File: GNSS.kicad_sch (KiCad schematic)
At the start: 0 parts

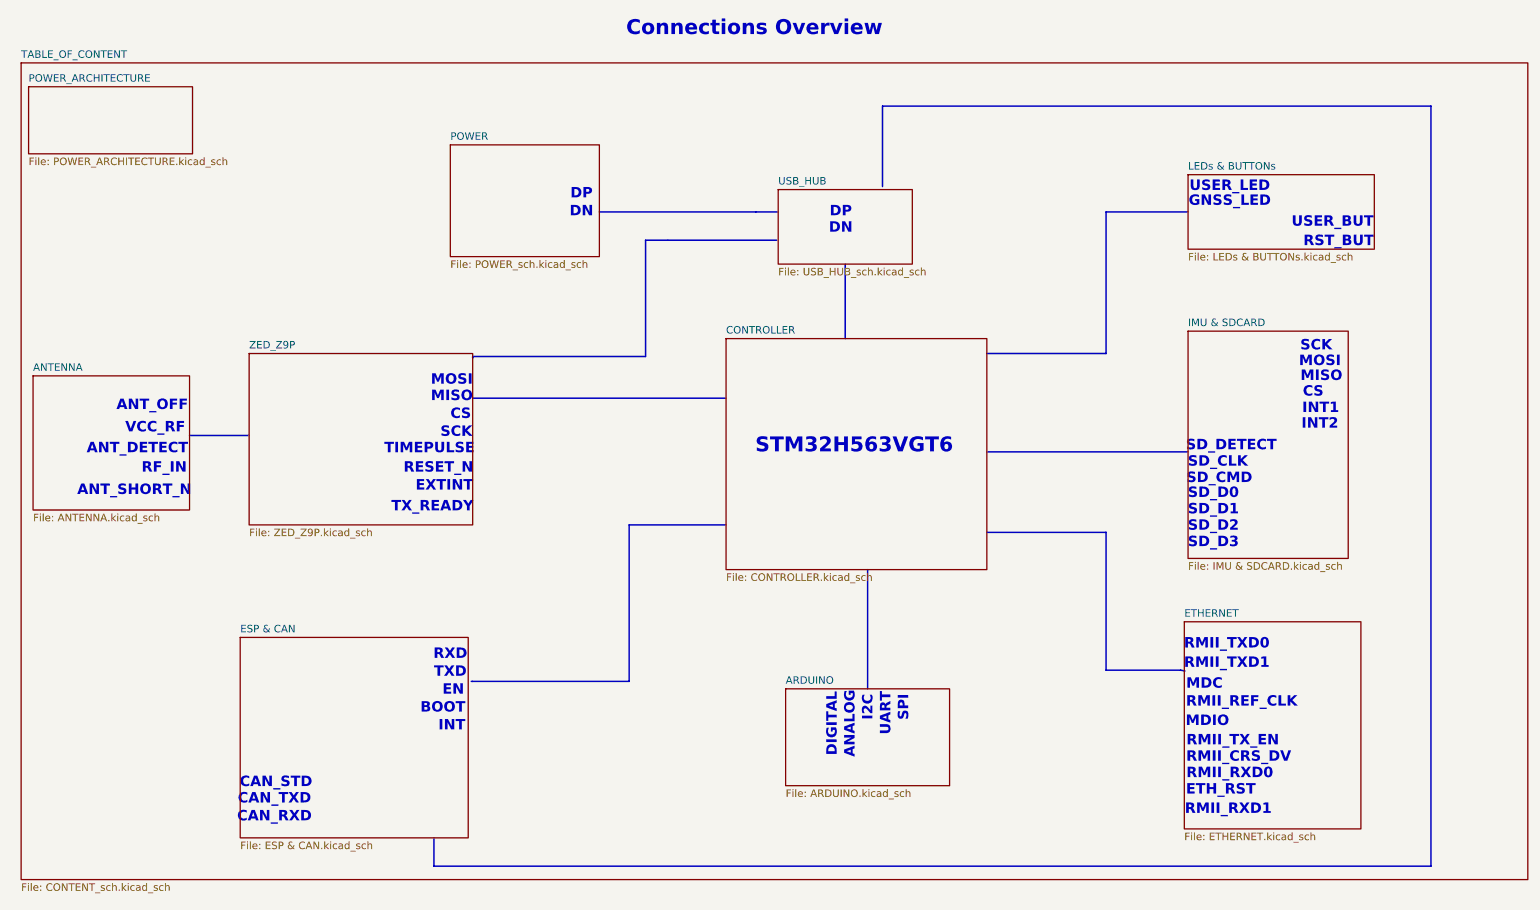
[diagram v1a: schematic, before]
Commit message: 18.09.2026
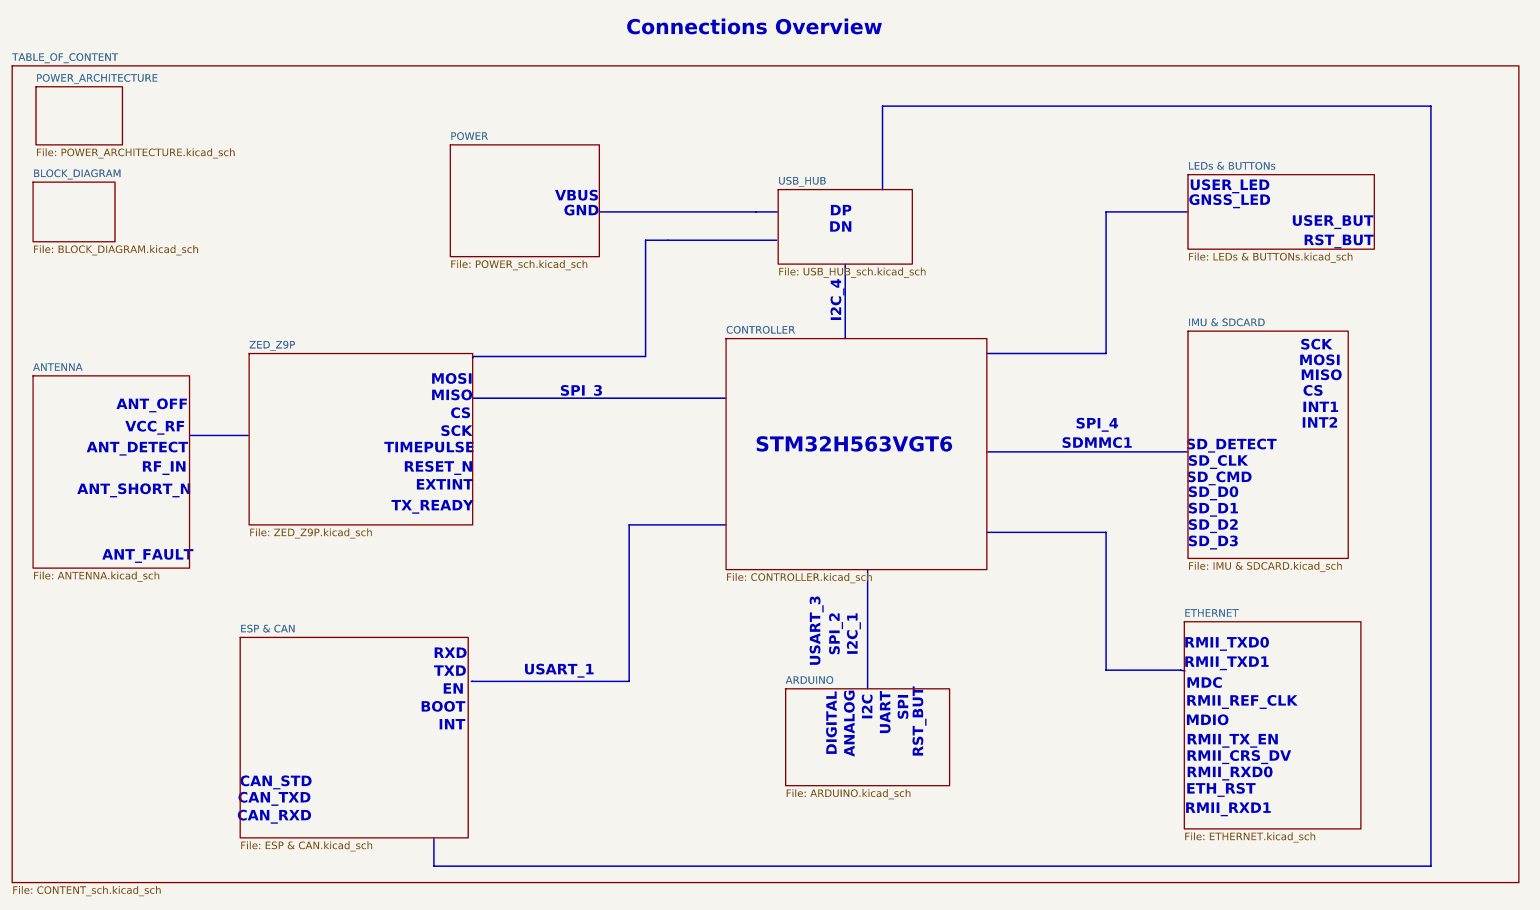
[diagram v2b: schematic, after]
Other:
- added sheet BLOCK_DIAGRAM (BLOCK_DIAGRAM.kicad_sch)
- note added: "ANT_FAULT"
- note added: "GND"
- note added: "I2C_1"
- note added: "I2C_4"
- note added: "SDMMC1"
- note added: "SPI_2"
- note added: "SPI_3"
- note added: "SPI_4"
- note added: "USART_1"
- note added: "USART_3"
- note added: "VBUS"
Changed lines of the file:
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@@
 	(polyline
 		(pts
-			(xy 167.64 45.212) (xy 167.64 31.496)
+			(xy 167.64 45.72) (xy 167.64 31.496)
 		)
 		(stroke
@@
 		)
 	)
-	(text "DP"
-		(exclude_from_sim no)
-		(at 116.332 46.482 0)
+	(text "VBUS"
+		(exclude_from_sim no)
+		(at 115.57 46.99 0)
 		(effects
 			(font
@@
 		)
 	)
+	(text "SPI_4"
+		(exclude_from_sim no)
+		(at 204.216 85.852 0)
+		(effects
+			(font
+				(size 1.778 1.778)
+				(bold yes)
+			)
+		)
+	)
 	(text "MISO"
 		(exclude_from_sim no)
@@
 		)
 	)
+	(text "I2C_1"
+		(exclude_from_sim no)
+		(at 162.56 121.666 90)
+		(effects
+			(font
+				(size 1.778 1.778)
+				(bold yes)
+			)
+		)
+	)
 	(text "TXD"
 		(exclude_from_sim no)
@@
 		(exclude_from_sim no)
 		(at 242.189 85.725 0)
+		(effects
+			(font
+				(size 1.778 1.778)
+				(bold yes)
+			)
+		)
+	)
+	(text "ANT_FAULT"
+		(exclude_from_sim no)
+		(at 42.418 108.204 0)
 		(effects
 			(font
@@
 		)
 	)
+	(text "SPI_2"
+		(exclude_from_sim no)
+		(at 159.512 121.666 90)
+		(effects
+			(font
+				(size 1.778 1.778)
+				(bold yes)
+			)
+		)
+	)
 	(text "DP"
 		(exclude_from_sim no)
@@
 		)
 	)
+	(text "RST_BUT"
+		(exclude_from_sim no)
+		(at 173.736 136.652 90)
+		(effects
+			(font
+				(size 1.778 1.778)
+				(bold yes)
+			)
+		)
+	)
 	(text "SD_D3"
 		(exclude_from_sim no)
@@
 		)
 	)
-	(text "DN"
+	(text "GND"
 		(exclude_from_sim no)
 		(at 116.332 49.53 0)
@@
 		)
 	)
+	(text "SDMMC1"
+		(exclude_from_sim no)
+		(at 204.216 89.154 0)
+		(effects
+			(font
+				(size 1.778 1.778)
+				(bold yes)
+			)
+		)
+	)
 	(text "RST_BUT"
 		(exclude_from_sim no)
@@
 		)
 	)
+	(text "USART_3"
+		(exclude_from_sim no)
+		(at 156.21 121.158 90)
+		(effects
+			(font
+				(size 1.778 1.778)
+				(bold yes)
+			)
+		)
+	)
 	(text "CAN_TXD"
 		(exclude_from_sim no)
@@
 		)
 	)
+	(text "SPI_3"
+		(exclude_from_sim no)
+		(at 116.332 80.264 0)
+		(effects
+			(font
+				(size 1.778 1.778)
+				(bold yes)
+			)
+		)
+	)
 	(text "MDIO"
 		(exclude_from_sim no)
@@
 		)
 	)
+	(text "I2C_4"
+		(exclude_from_sim no)
+		(at 159.766 64.77 90)
+		(effects
+			(font
+				(size 1.778 1.778)
+				(bold yes)
+			)
+		)
+	)
+	(text "USART_1"
+		(exclude_from_sim no)
+		(at 112.522 127.762 0)
+		(effects
+			(font
+				(size 1.778 1.778)
+				(bold yes)
+			)
+		)
+	)
 	(text "INT1"
 		(exclude_from_sim no)
@@
 	)
 	(sheet
-		(at 20.828 24.13)
+		(at 19.304 24.638)
 		(size 256.794 139.192)
 		(fields_autoplaced yes)
@@
 		)
 		(property "Sheetname" "TABLE_OF_CONTENT"
-			(at 20.828 23.4184 0)
+			(at 19.304 23.9264 0)
 			(effects
 				(font
@@
 		)
 		(property "Sheetfile" "CONTENT_sch.kicad_sch"
-			(at 20.828 163.9066 0)
+			(at 19.304 164.4146 0)
 			(effects
 				(font
@@
 	)
 	(sheet
+		(at 22.86 44.45)
+		(size 13.97 10.16)
+		(fields_autoplaced yes)
+		(stroke
+			(width 0.1524)
+			(type solid)
+		)
+		(fill
+			(color 0 0 0 0.0000)
+		)
+		(property "Sheetname" "BLOCK_DIAGRAM"
+			(at 22.86 43.7384 0)
+			(effects
+				(font
+					(size 1.27 1.27)
+				)
+				(justify left bottom)
+			)
+		)
+		(property "Sheetfile" "BLOCK_DIAGRAM.kicad_sch"
+			(at 22.86 55.1946 0)
+			(effects
+				(font
+					(size 1.27 1.27)
+				)
+				(justify left top)
+			)
+		)
+		(instances
+			(project "GNSS"
+				(path "/a70dad34-b24c-4b58-b91c-f14576b5da7d"
+					(page "15")
+				)
+			)
+		)
+	)
+	(sheet
 		(at 59.69 73.66)
 		(size 38.1 29.21)
@@
 	)
 	(sheet
-		(at 22.098 28.194)
-		(size 27.94 11.43)
+		(at 23.368 28.194)
+		(size 14.732 9.906)
 		(fields_autoplaced yes)
 		(stroke
@@
 		)
 		(property "Sheetname" "POWER_ARCHITECTURE"
-			(at 22.098 27.4824 0)
+			(at 23.368 27.4824 0)
 			(effects
 				(font
@@
 		)
 		(property "Sheetfile" "POWER_ARCHITECTURE.kicad_sch"
-			(at 22.098 40.2086 0)
+			(at 23.368 38.6846 0)
 			(effects
 				(font
@@
 	(sheet
 		(at 22.86 77.47)
-		(size 26.67 22.86)
+		(size 26.67 32.766)
 		(fields_autoplaced yes)
 		(stroke
@@
 		)
 		(property "Sheetfile" "ANTENNA.kicad_sch"
-			(at 22.86 100.9146 0)
-			(effects
-				(font
+			(at 22.86 110.8206 0)
+			(effects
+				(font
